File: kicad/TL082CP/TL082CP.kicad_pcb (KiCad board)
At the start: 2 copper layers, 80 x 100 mm, 16 parts, among them J1 AudioJack2_Switch, J2 AudioJack2_Switch, J4 Barrel_Jack, U1 TMR_1-1222, U2 TL082

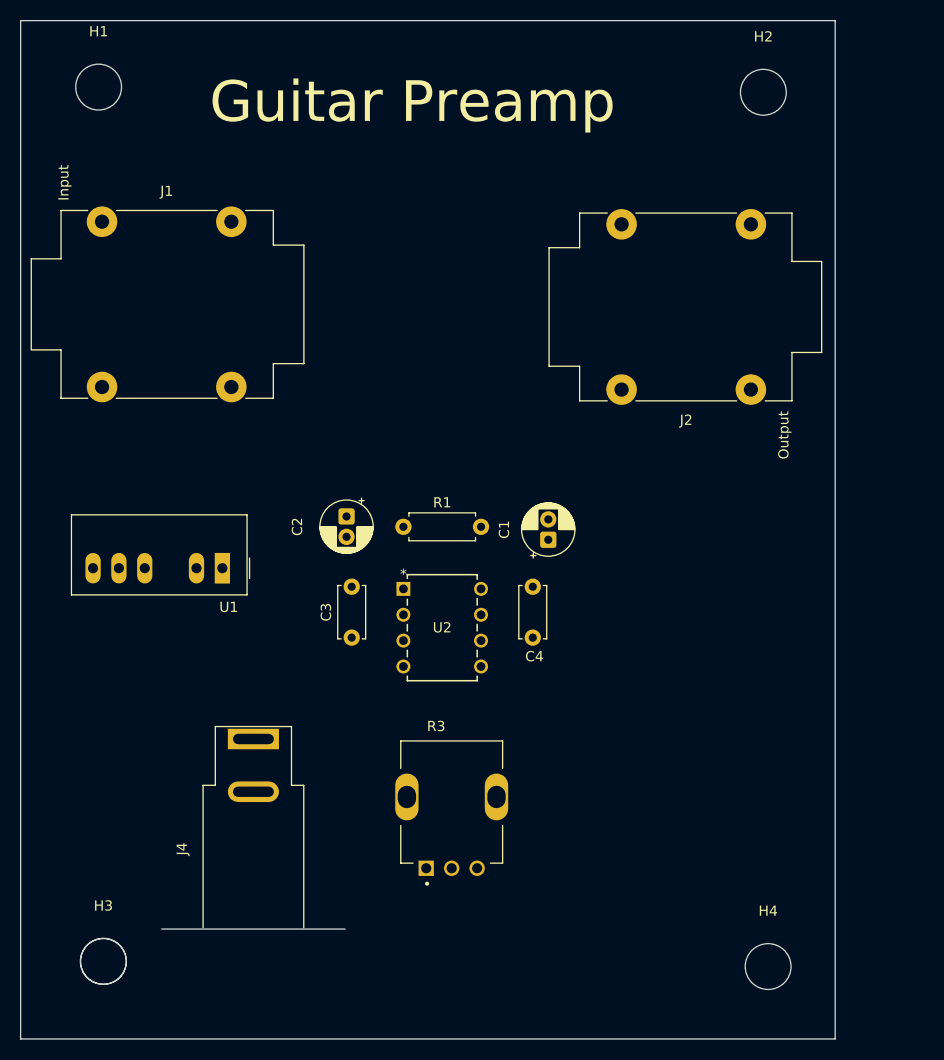
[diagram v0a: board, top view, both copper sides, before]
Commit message: feat: pcb routing
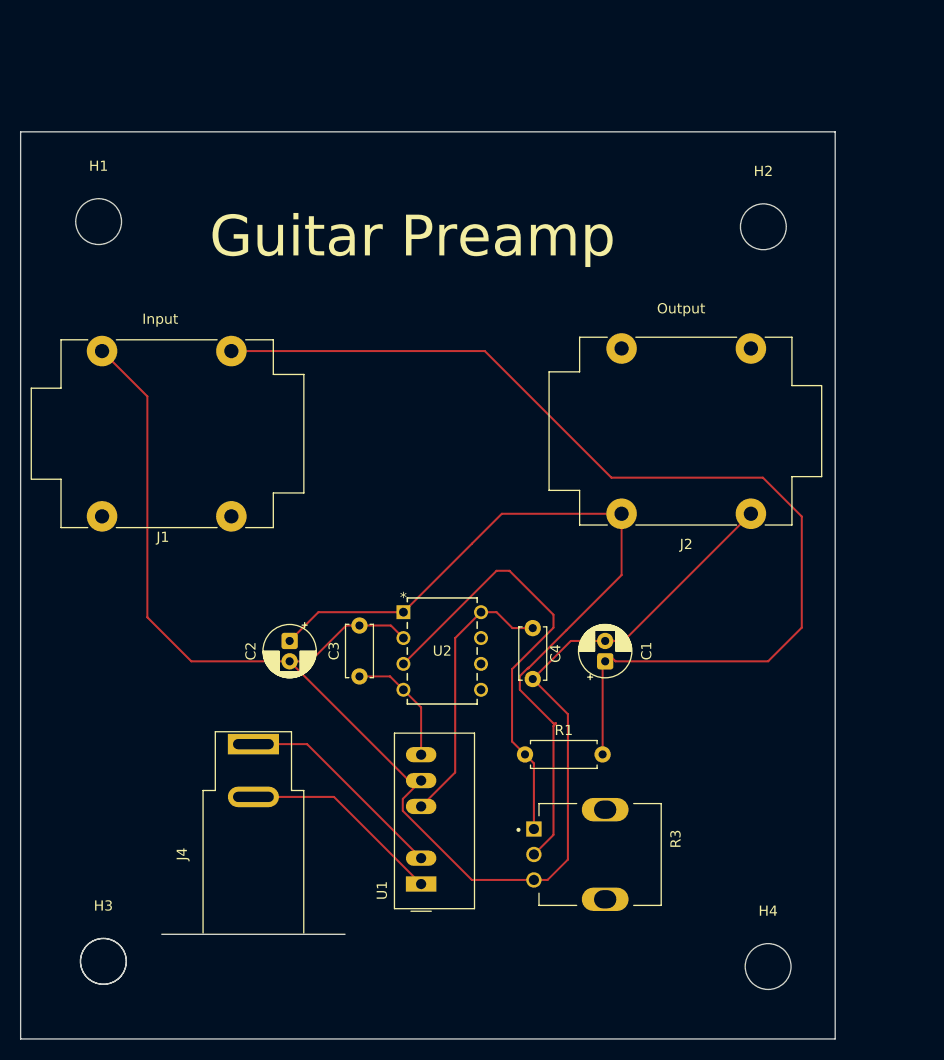
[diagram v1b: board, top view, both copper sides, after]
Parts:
- moved U1 36.6 mm to (133.9, 113.3), turned to 90 degrees
- moved R1 25.3 mm to (144.1, 100.6)
- moved R3 16.1 mm to (152.0, 110.4), turned to -90 degrees
- moved C2 13.4 mm to (121.0, 89.4)
- moved H1 13.2 mm to (102.3, 48.3)
- moved H2 13.2 mm to (167.6, 48.8)
- moved C1 13.2 mm to (152.0, 91.4)
- moved J1 12.7 mm to (102.6, 61.0)
- moved J2 12.2 mm to (166.3, 76.9)
- moved C4 4.06 mm to (144.9, 88.2)
- moved C3 3.89 mm to (127.9, 92.9)
- moved U2 2.29 mm to (132.2, 86.6)
- moved J4 0.51 mm to (117.5, 99.6)
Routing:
- net GND: track 0.00 -> 145.8 mm
- net /audio_signal/Audio-IN: track 0.00 -> 103.9 mm
- net /audio_signal/Audio-OUT: track 0.00 -> 78.1 mm
- net Net-(U2A-+): track 0.00 -> 43.9 mm
- net +12V: track 0.00 -> 27.2 mm
- net /dual supply voltage/+VIN: track 0.00 -> 21.1 mm
- net /dual supply voltage/-VIN: track 0.00 -> 20.0 mm
- net -12V: track 0.00 -> 12.0 mm
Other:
- board size 80 x 100 mm -> 80 x 89.1 mm
- board text added: "C1"
- board text added: "C4"

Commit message: final pcb layout and updated doc
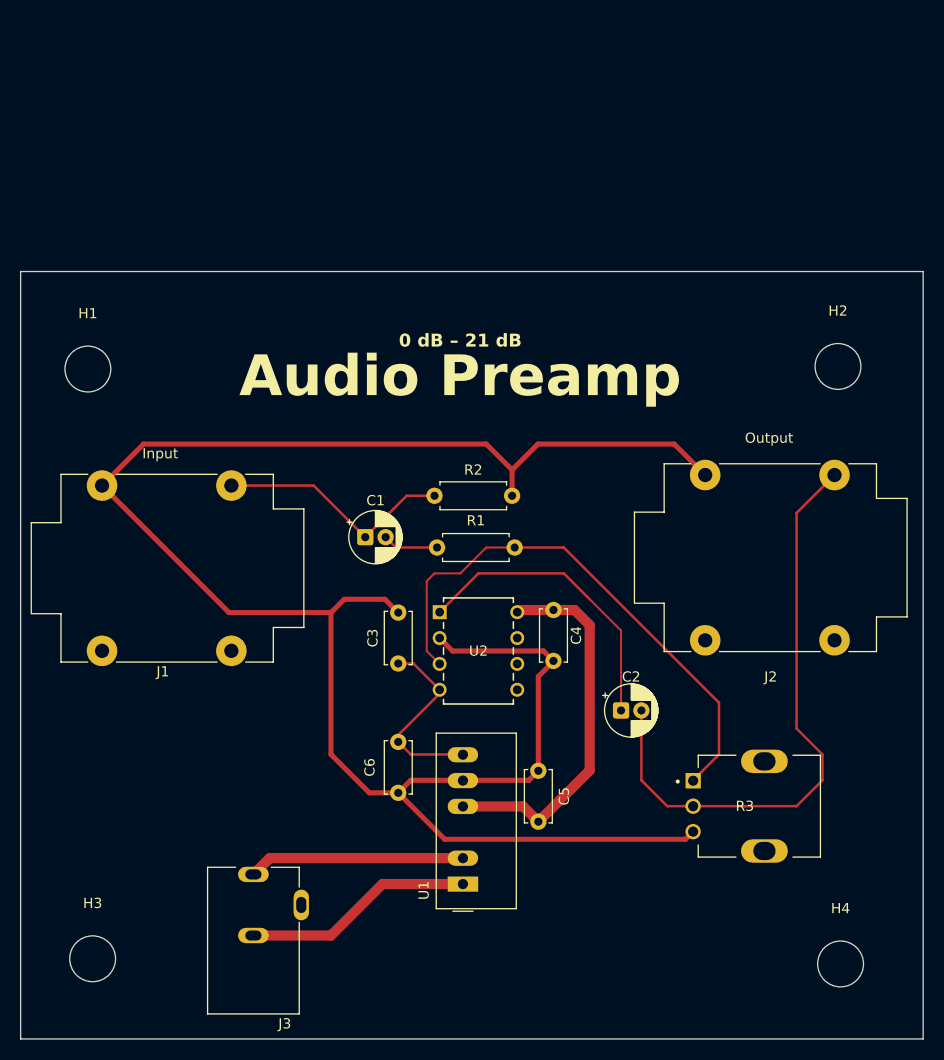
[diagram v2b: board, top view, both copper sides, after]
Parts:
- removed ?: , 
- removed J4: Barrel_Jack, Connector_BarrelJack:BarrelJack_SwitchcraftConxall_RAPC10U_Horizontal
- added C5: 100nF, Capacitor_THT:C_Disc_D5.0mm_W2.5mm_P5.00mm, F.Cu at (145.5, 107.2)
- added C6: 100nF, Capacitor_THT:C_Disc_D5.0mm_W2.5mm_P5.00mm, F.Cu at (131.7, 99.4)
- added J3: PJ-102A, 1_own_PJ-102A:CUI_PJ-102A, F.Cu at (117.5, 115.4)
- added R2: 1Meg, Resistor_THT:R_Axial_DIN0207_L6.3mm_D2.5mm_P7.62mm_Horizontal, F.Cu at (135.3, 75.2)
- R1: value 1k -> 4,7k
- moved C2 33.3 mm to (153.6, 96.3), turned to 0 degrees
- moved C1 26.5 mm to (128.5, 79.2), turned to 0 degrees
- moved R1 20.3 mm to (143.1, 80.3), turned to 180 degrees
- moved R3 16.3 mm to (167.7, 105.7)
- moved H2 15.6 mm to (174.9, 62.5)
- moved H1 14.5 mm to (101.2, 62.7)
- moved J1 13.2 mm to (102.6, 74.2)
- moved H4 7.12 mm to (175.1, 121.2)
- moved J2 5.88 mm to (161.8, 73.1), turned to 0 degrees
- moved U1 4.10 mm to (138.0, 113.3)
- moved C3 4.02 mm to (131.7, 91.7)
- moved U2 3.56 mm to (135.8, 86.6)
- moved C4 2.70 mm to (146.9, 86.4)
- moved H3 1.09 mm to (101.7, 120.7)
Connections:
- C1 pad 2: GND -> Net-(C1-Pad2)
- C2 pad 1: /audio_signal/Audio-OUT -> Net-(U2A-OUT)
- C2 pad 2: GND -> /audio_signal/Audio-OUT
- R1 pad 2: /audio_signal/Audio-IN -> Net-(C1-Pad2)
- U2 pad 1: /audio_signal/Audio-OUT -> Net-(U2A-OUT)
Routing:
- net /audio_signal/Audio-IN: track 103.9 -> 23.7 mm
- net GND: track 145.8 -> 193.6 mm
- net Net-(U2A-OUT): track 0.00 -> 29.6 mm
- net /audio_signal/Audio-OUT: track 78.1 -> 59.3 mm
- net +12V: track 27.2 -> 37.2 mm
- net Net-(U2A-+): track 43.9 -> 53.8 mm
- net -12V: track 12.0 -> 18.8 mm
- net Net-(C1-Pad2): track 0.00 -> 5.47 mm
- net /dual supply voltage/-VIN: track 20.0 -> 22.7 mm
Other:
- board size 80 x 89.1 mm -> 88.6 x 75.4 mm
- board text added: "0 dB – 21 dB"
- board text added: "Audio Preamp"
- board text removed: "Guitar Preamp"
